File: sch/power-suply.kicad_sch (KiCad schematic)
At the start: 38 parts, among them J5 12V_in, Q2 DMT6007LFG-7, U1 LMR51450SDRRR, U2 LM74700QDBVTQ1, U3 LMR51450SDRRR

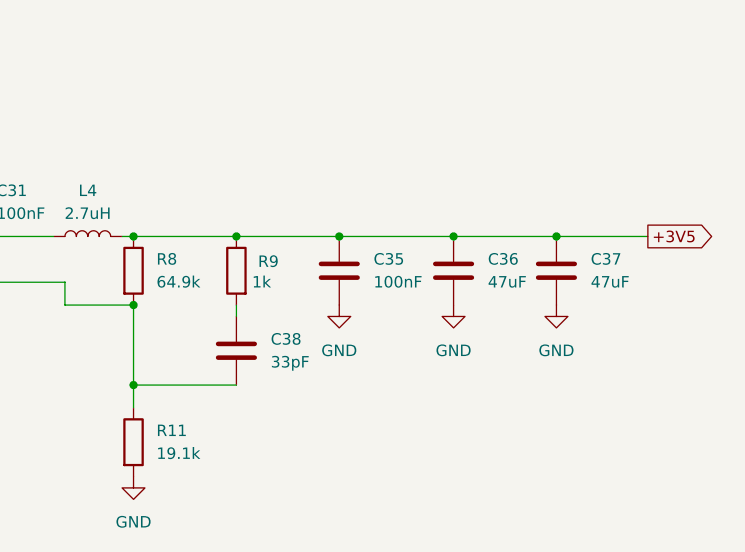
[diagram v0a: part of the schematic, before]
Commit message: Homestretch
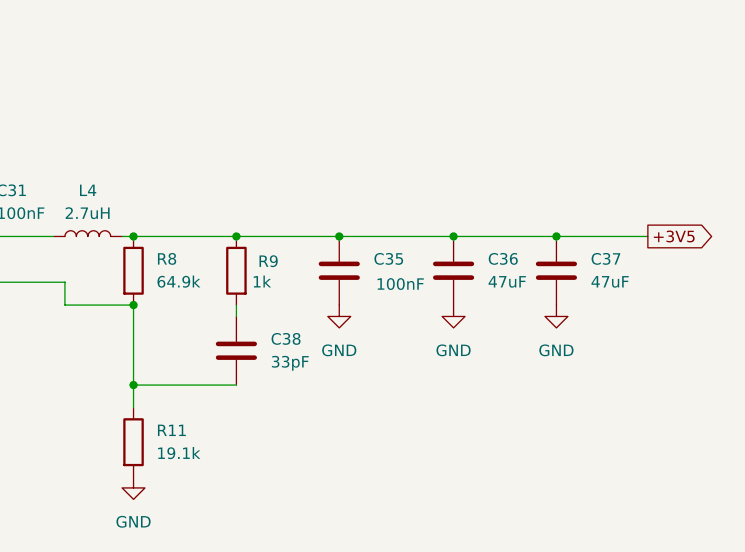
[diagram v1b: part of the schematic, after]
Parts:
- R8: footprint Resistor_SMD:R_0201_0603Metric -> Resistor_SMD:R_0603_1608Metric
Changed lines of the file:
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@@
 		)
 		(property "Value" "100nF"
-			(at 245.11 99.0599 0)
+			(at 245.364 99.314 0)
 			(effects
 				(font
@@
 			)
 		)
-		(property "Footprint" "Resistor_SMD:R_0201_0603Metric"
+		(property "Footprint" "Resistor_SMD:R_0603_1608Metric"
 			(at 216.662 97.79 90)
 			(effects
